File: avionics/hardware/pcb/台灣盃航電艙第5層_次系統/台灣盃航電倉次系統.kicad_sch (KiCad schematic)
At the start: 54 parts, among them J1 SH 1.0, J2 Micro_SD_Card, J3 SMA, J4 SMA, J5 Conn_01x04_Pin, J6 Conn_01x06_Pin, SW2 SW_SPST, U1 STM32F103C8Tx, U2 BMP390L, U3 NEO-M9N, U6 E22-400T22S, Y1 8MHz

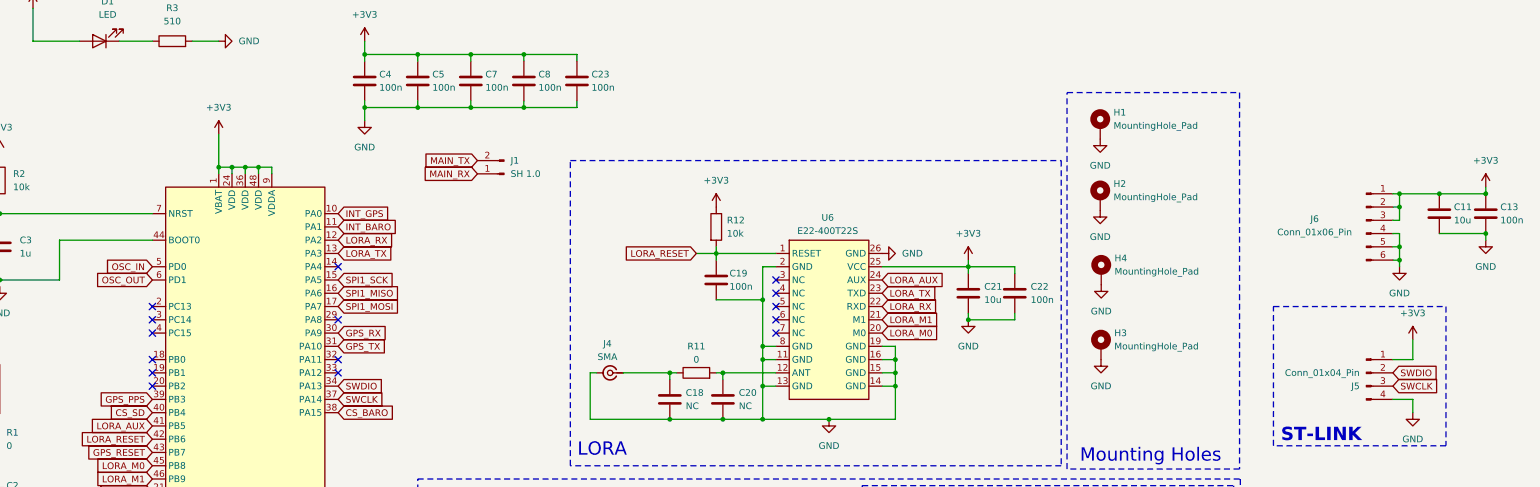
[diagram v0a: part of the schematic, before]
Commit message: 完成PCB最終設計
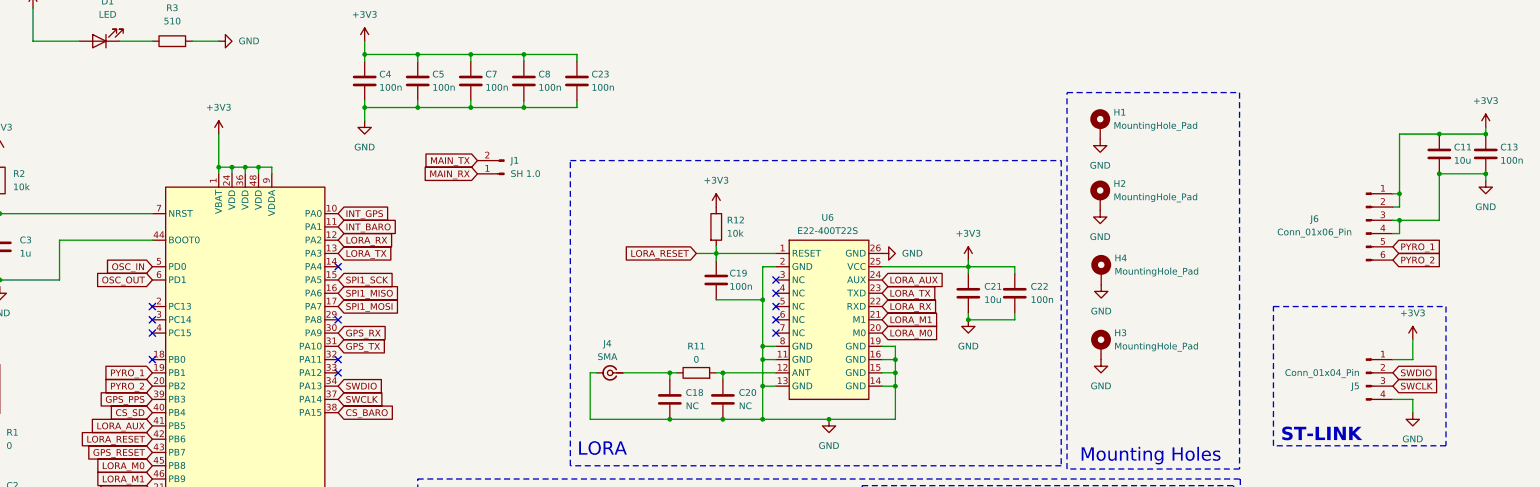
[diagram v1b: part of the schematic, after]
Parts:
- J3, J4: footprint Connector_Coaxial:SMA_Amphenol_132134-10_Vertical -> Connector_Coaxial:SMA_Amphenol_132134-11_Vertical
- U6: footprint E22-900T22S:E22-900T22S -> E22-900T22S:PE22-230T22S
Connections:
- net +3V3: no longer J6.3 (Pin_3)
- net GND: now also J6.3 (Pin_3); no longer J6.5 (Pin_5), J6.6 (Pin_6)
- net PYRO_1: now reaches U1.19 (PB1)
- net PYRO_1: now also J6.5 (Pin_5)
- net PYRO_2: now reaches U1.20 (PB2)
- net PYRO_2: now also J6.6 (Pin_6)
- no-connect marks 22 -> 20
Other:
- moved on the sheet: C11, C13
